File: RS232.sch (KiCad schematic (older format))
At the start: 1 part

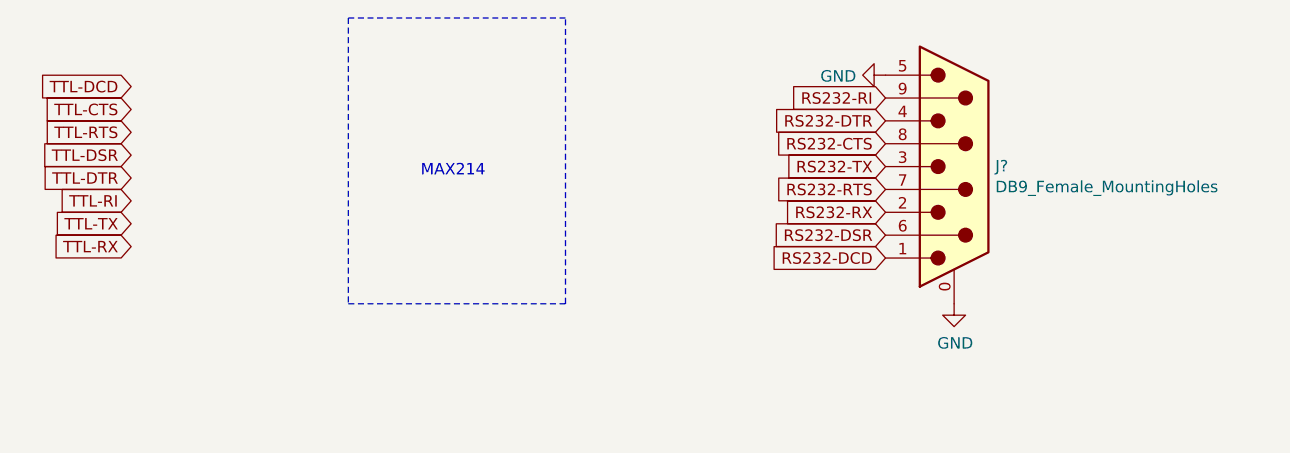
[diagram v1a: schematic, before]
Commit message: updates
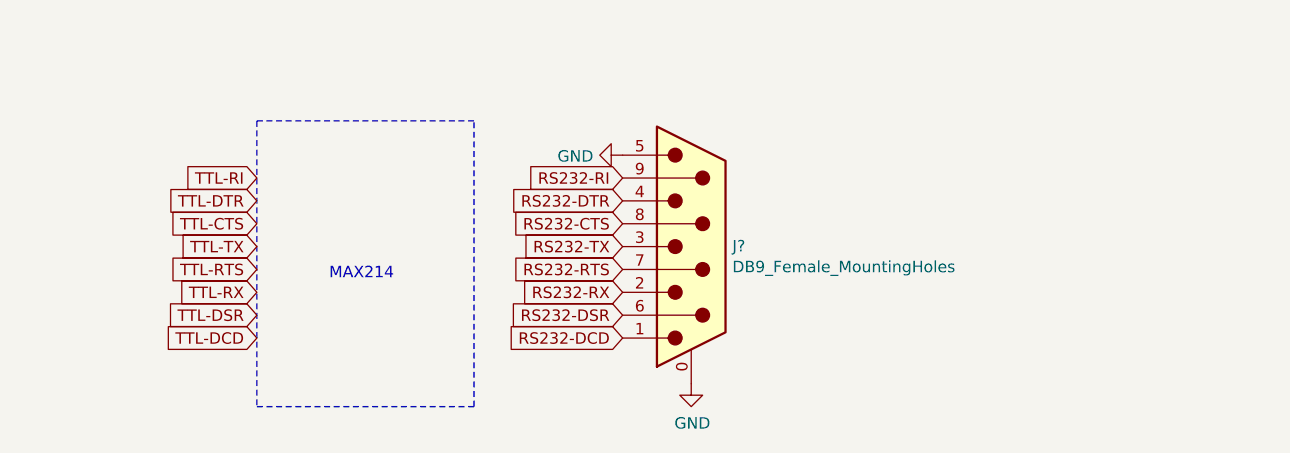
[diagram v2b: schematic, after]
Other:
- moved on the sheet: J?
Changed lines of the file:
@@
 L Connector:DB9_Male_MountingHoles J?
 U 1 1 60ECC003
-P 7750 3600
-F 0 "J?" H 7930 3602 50  0000 L CNN
-F 1 "DB9_Female_MountingHoles" H 7930 3511 50  0000 L CNN
-F 2 "" H 7750 3600 50  0001 C CNN
-F 3 " ~" H 7750 3600 50  0001 C CNN
-	1    7750 3600
+P 6600 3950
+F 0 "J?" H 6780 3952 50  0000 L CNN
+F 1 "DB9_Female_MountingHoles" H 6780 3861 50  0000 L CNN
+F 2 "" H 6600 3950 50  0001 C CNN
+F 3 " ~" H 6600 3950 50  0001 C CNN
+	1    6600 3950
 	1    0    0    -1
 $EndComp
-Text GLabel 4150 3650 0    50   Input ~ 0
+Text GLabel 4700 3750 0    50   Input ~ 0
 TTL-DTR
-Text GLabel 4150 3550 0    50   Input ~ 0
+Text GLabel 4700 4250 0    50   Input ~ 0
 TTL-DSR
-Text GLabel 4150 3850 0    50   Input ~ 0
+Text GLabel 4700 3950 0    50   Input ~ 0
 TTL-TX
-Text GLabel 4150 3950 0    50   Input ~ 0
+Text GLabel 4700 4150 0    50   Input ~ 0
 TTL-RX
-Text GLabel 4150 3750 0    50   Input ~ 0
+Text GLabel 4700 3650 0    50   Input ~ 0
 TTL-RI
-Text GLabel 7450 3700 0    50   Input ~ 0
+Text GLabel 6300 4050 0    50   Input ~ 0
 RS232-RTS
-Text GLabel 7450 3500 0    50   Input ~ 0
+Text GLabel 6300 3850 0    50   Input ~ 0
 RS232-CTS
-Text GLabel 7450 3400 0    50   Input ~ 0
+Text GLabel 6300 3750 0    50   Input ~ 0
 RS232-DTR
-Text GLabel 7450 3900 0    50   Input ~ 0
+Text GLabel 6300 4250 0    50   Input ~ 0
 RS232-DSR
-Text GLabel 7450 3600 0    50   Input ~ 0
+Text GLabel 6300 3950 0    50   Input ~ 0
 RS232-TX
-Text GLabel 7450 3800 0    50   Input ~ 0
+Text GLabel 6300 4150 0    50   Input ~ 0
 RS232-RX
-Text GLabel 7450 4000 0    50   Input ~ 0
+Text GLabel 6300 4350 0    50   Input ~ 0
 RS232-DCD
-Text GLabel 7450 3300 0    50   Input ~ 0
+Text GLabel 6300 3650 0    50   Input ~ 0
 RS232-RI
 $Comp
 L power:GND #PWR?
 U 1 1 60ED1EA7
-P 7750 4200
-F 0 "#PWR?" H 7750 3950 50  0001 C CNN
-F 1 "GND" H 7755 4027 50  0000 C CNN
-F 2 "" H 7750 4200 50  0001 C CNN
-F 3 "" H 7750 4200 50  0001 C CNN
-	1    7750 4200
+P 6600 4550
+F 0 "#PWR?" H 6600 4300 50  0001 C CNN
+F 1 "GND" H 6605 4377 50  0000 C CNN
+F 2 "" H 6600 4550 50  0001 C CNN
+F 3 "" H 6600 4550 50  0001 C CNN
+	1    6600 4550
 	1    0    0    -1
 $EndComp
@@
 L power:GND #PWR?
 U 1 1 60ED3990
-P 7450 3200
-F 0 "#PWR?" H 7450 2950 50  0001 C CNN
-F 1 "GND" V 7455 3072 50  0000 R CNN
-F 2 "" H 7450 3200 50  0001 C CNN
-F 3 "" H 7450 3200 50  0001 C CNN
-	1    7450 3200
+P 6300 3550
+F 0 "#PWR?" H 6300 3300 50  0001 C CNN
+F 1 "GND" V 6305 3422 50  0000 R CNN
+F 2 "" H 6300 3550 50  0001 C CNN
+F 3 "" H 6300 3550 50  0001 C CNN
+	1    6300 3550
 	0    1    1    0
 $EndComp
 Wire Notes Line
-	5100 2950 5100 4200
+	4700 3400 4700 4650
 Wire Notes Line
-	5100 4200 6050 4200
+	4700 4650 5650 4650
 Wire Notes Line
-	6050 4200 6050 2950
+	5650 4650 5650 3400
 Wire Notes Line
-	6050 2950 5100 2950
-Text Notes 5700 3650 2    50   ~ 0
+	5650 3400 4700 3400
+Text Notes 5300 4100 2    50   ~ 0
 MAX214
-Text GLabel 4150 3250 0    50   Input ~ 0
+Text GLabel 4700 4350 0    50   Input ~ 0
 TTL-DCD
-Text GLabel 4150 3350 0    50   Input ~ 0
+Text GLabel 4700 3850 0    50   Input ~ 0
 TTL-CTS
-Text GLabel 4150 3450 0    50   Input ~ 0
+Text GLabel 4700 4050 0    50   Input ~ 0
 TTL-RTS
 $EndSCHEMATC

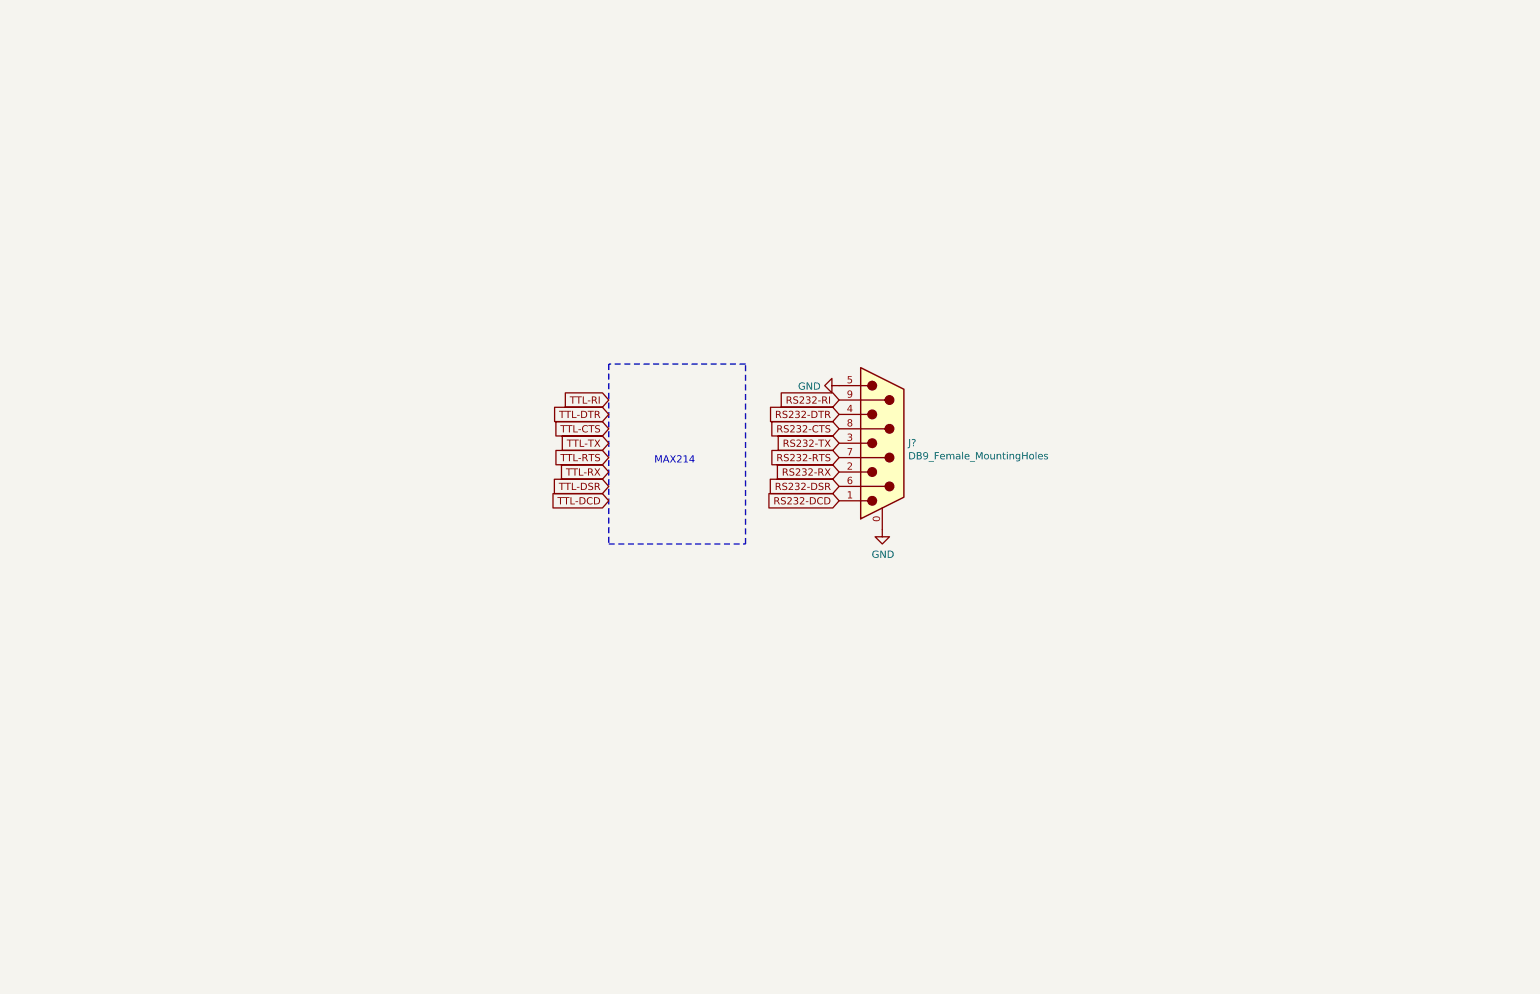
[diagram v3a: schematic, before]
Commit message: updates
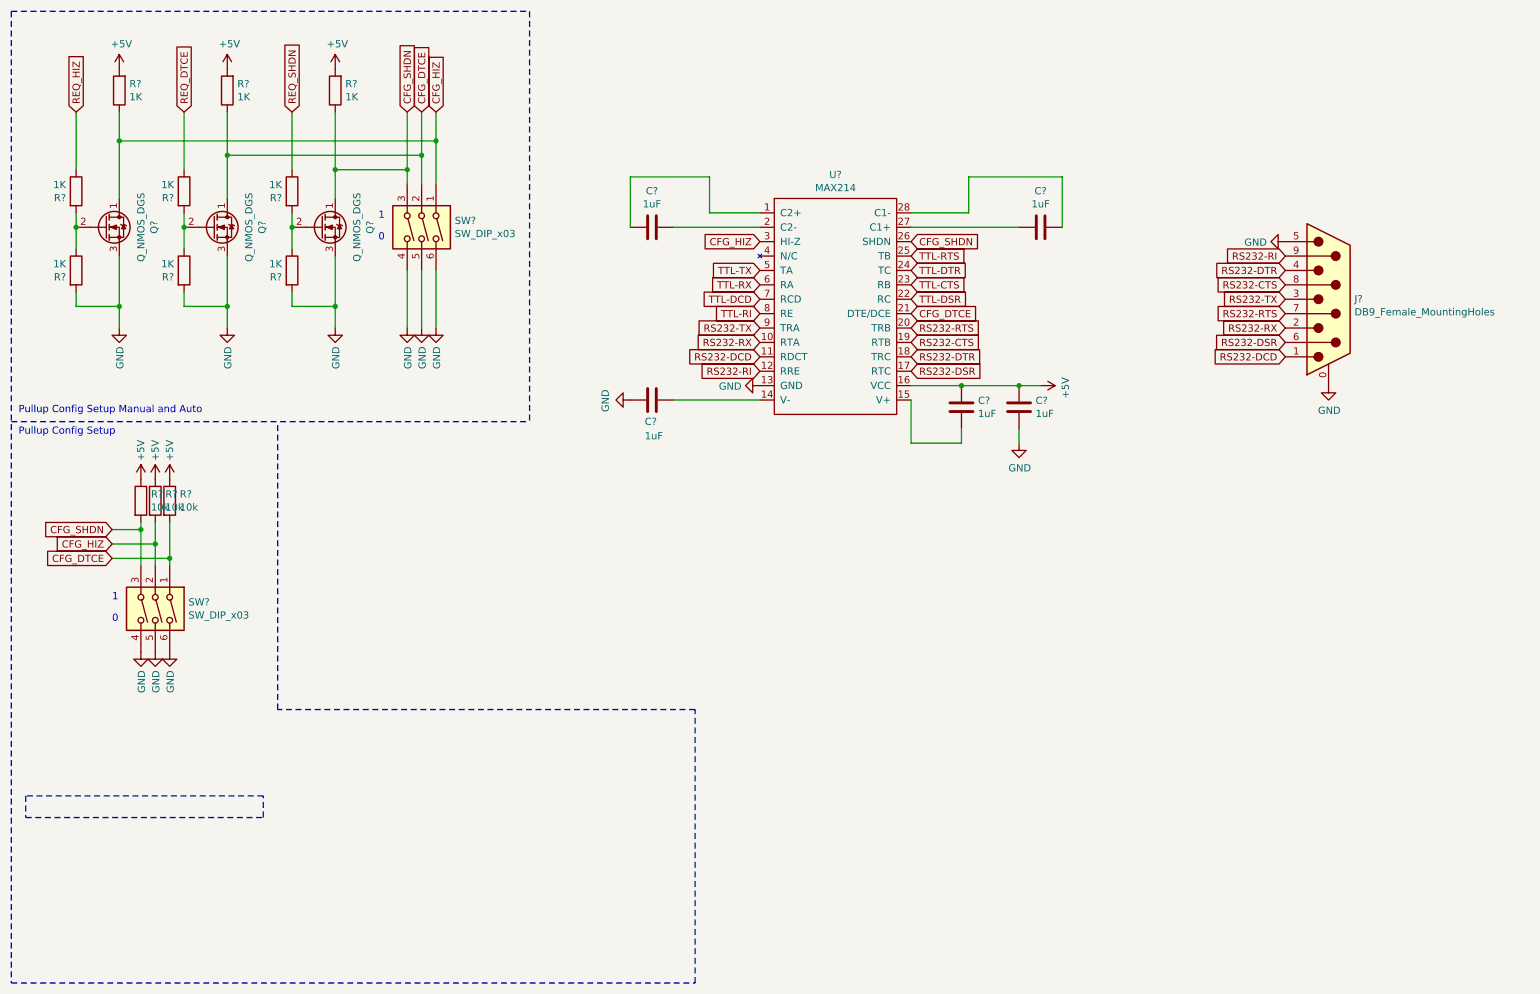
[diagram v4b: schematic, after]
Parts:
- added C? (x5): 1uF, symbol Device:C
- added Q? (x3): Q_NMOS_DGS, symbol Device:Q_NMOS_DGS
- added R? (x3): 10k, symbol Device:R
- added R? (x9): 1K, symbol Device:R
- added SW? (x2): SW_DIP_x03, symbol Switch:SW_DIP_x03
- added U?: MAX214, symbol Sebs:MAX214
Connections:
- net GND: now also C?.2, C?.2, Q?.3 (S), Q?.3 (S), Q?.3 (S), R?.2, R?.2, R?.2, SW?.4, SW?.4, SW?.5, SW?.5, SW?.6, SW?.6, U?.13 (GND)
- net RS232-CTS: now also U?.19 (RTB)
- net RS232-DCD: now also U?.11 (RDCT)
- net RS232-DSR: now also U?.17 (RTC)
- net RS232-DTR: now also U?.18 (TRC)
- net RS232-RI: now also U?.12 (RRE)
- net RS232-RTS: now also U?.20 (TRB)
- net RS232-RX: now also U?.10 (RTA)
- net RS232-TX: now also U?.9 (TRA)
- net TTL-CTS: now also U?.23 (RB)
- net TTL-DCD: now also U?.7 (RCD)
- net TTL-DSR: now also U?.22 (RC)
- net TTL-DTR: now also U?.24 (TC)
- net TTL-RI: now also U?.8 (RE)
- net TTL-RTS: now also U?.25 (TB)
- net TTL-RX: now also U?.6 (RA)
- net TTL-TX: now also U?.5 (TA)
- new net: C?.2, U?.1 (C2+)
- new net: C?.1, U?.14 (V-)
- new net: C?.1, U?.15 (V+)
- new net: C?.1, U?.2 (C2-)
- new net: C?.2, U?.27 (C1+)
- new net: C?.1, U?.28 (C1-)
- new net: Q?.2 (G), R?.1, R?.2 (x3)
- new net +5V: C?.1, C?.2, R?.1, R?.1, R?.1, R?.2, R?.2, R?.2, U?.16 (VCC)
- new net CFG_DTCE: Q?.1 (D), R?.1, R?.2, SW?.1, SW?.2, U?.21 (DTE/DCE)
- new net CFG_HIZ: Q?.1 (D), R?.1, R?.2, SW?.1, SW?.2, U?.3 (HI-Z)
- new net CFG_SHDN: Q?.1 (D), R?.1, R?.2, SW?.3, SW?.3, U?.26 (SHDN)
- new net REQ_DTCE: R?.1
- new net REQ_HIZ: R?.1
- new net REQ_SHDN: R?.1
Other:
- note added: "0"
- note added: "1"
- note added: "Pullup Config Setup"
- note added: "Pullup Config Setup Manual and Auto"
- note removed: "MAX214"
- moved on the sheet: J?
